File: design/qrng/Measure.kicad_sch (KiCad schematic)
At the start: 5 parts

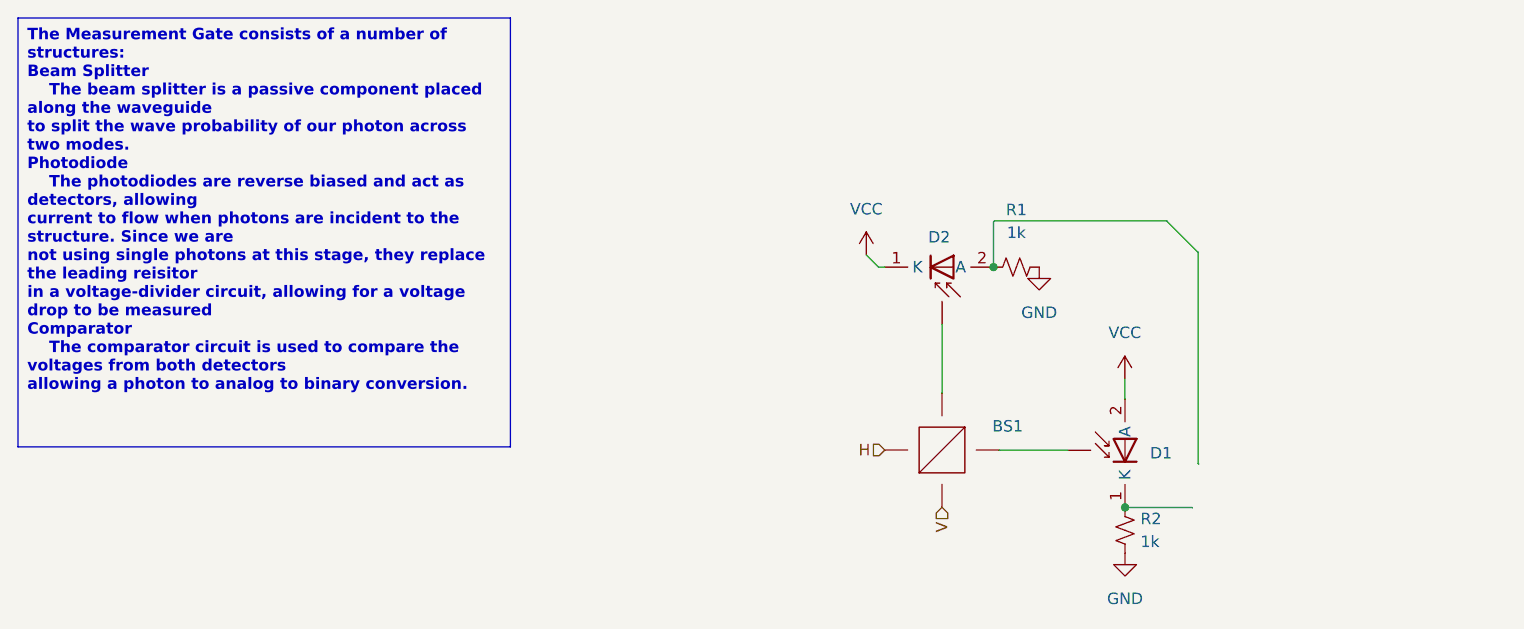
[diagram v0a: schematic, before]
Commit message: Updated KiCAD design
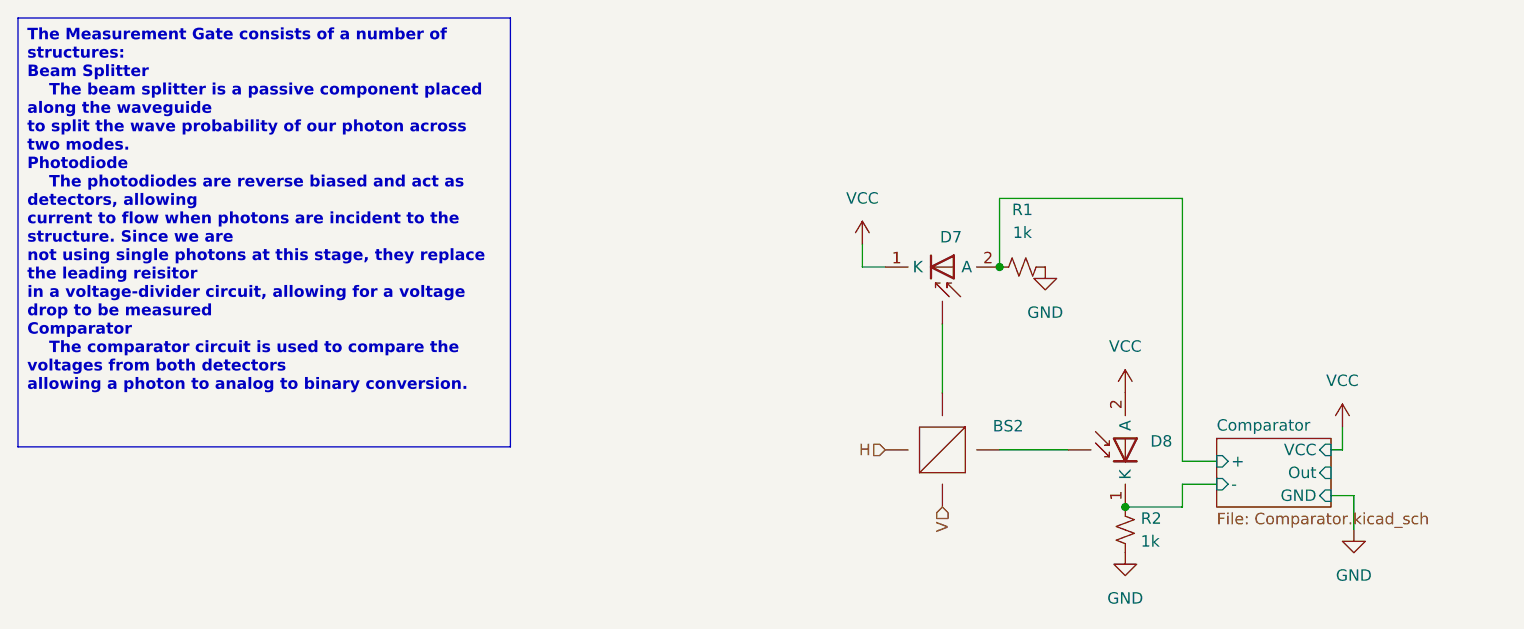
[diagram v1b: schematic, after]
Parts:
- renumbered BS1 to BS2, D2 to D7, D1 to D8
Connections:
- net Comparator/-: now reaches D8.1 (K), R2.2
- net Comparator/+: now reaches D7.2 (A), R1.1
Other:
- added sheet Comparator (Comparator.kicad_sch)
- moved on the sheet: R1
